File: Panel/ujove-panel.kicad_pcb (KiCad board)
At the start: 2 copper layers, 40.3 x 128.5 mm, 0 parts

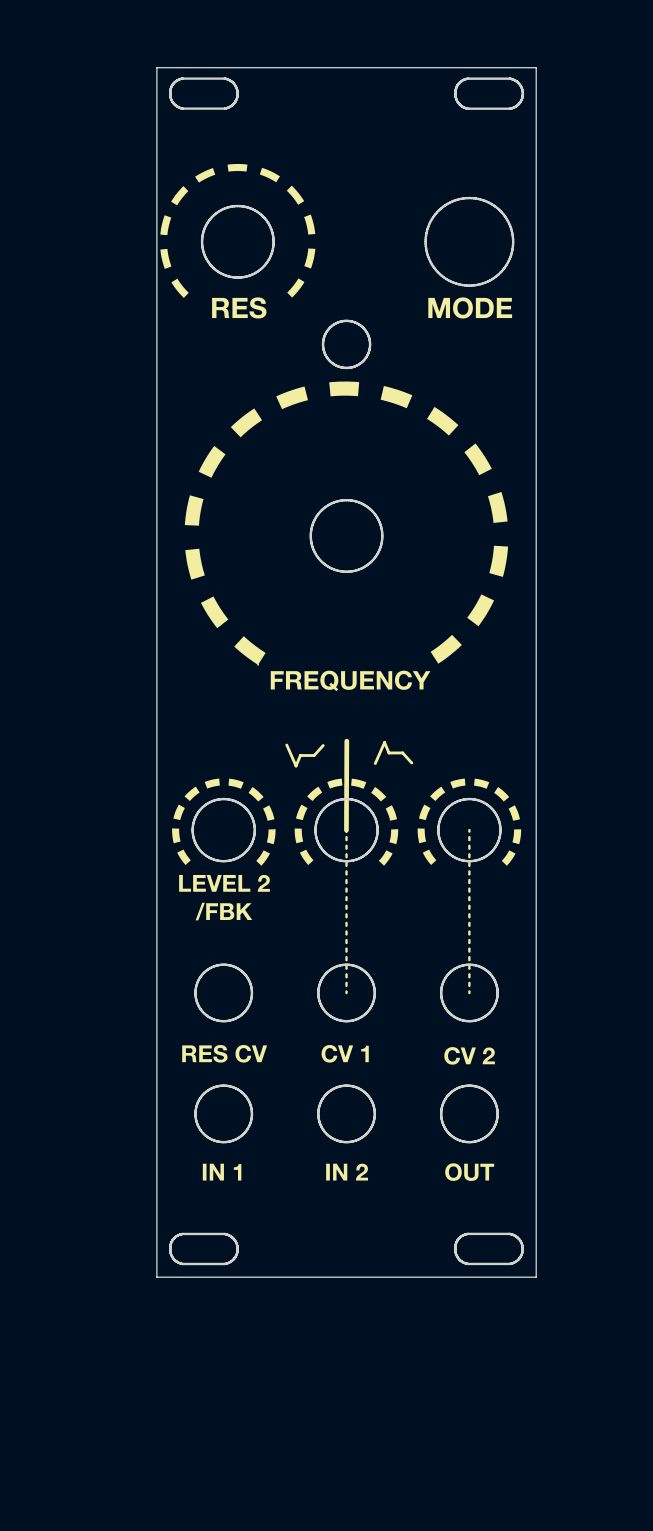
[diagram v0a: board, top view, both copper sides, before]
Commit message: Add files via upload
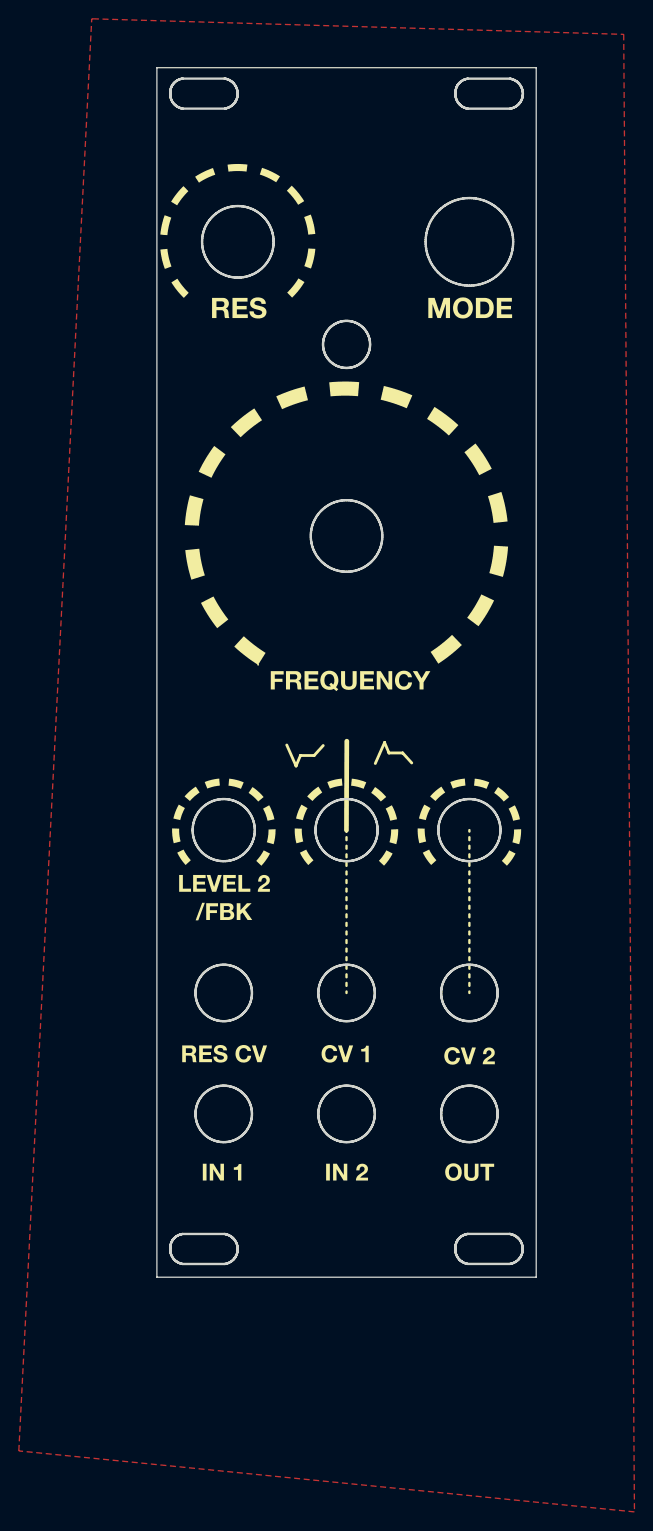
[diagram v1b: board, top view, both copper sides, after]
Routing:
- added copper zone on F.Cu, net (none)
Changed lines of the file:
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@@
 		(layer "Edge.Cuts")
 	)
+	(zone
+		(net 0)
+		(net_name "")
+		(layer "F.Cu")
+		(hatch edge 0.5)
+		(connect_pads
+			(clearance 0.5)
+		)
+		(min_thickness 0.25)
+		(filled_areas_thickness no)
+		(fill yes
+			(thermal_gap 0.5)
+			(thermal_bridge_width 0.5)
+			(island_removal_mode 1)
+			(island_area_min 10)
+		)
+		(polygon
+			(pts
+				(xy 46.101 25.019) (xy 102.489 26.67) (xy 103.632 183.642) (xy 38.227 177.165) (xy 45.974 25.019)
+			)
+		)
+	)
 )
